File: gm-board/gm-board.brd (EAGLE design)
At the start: 59.5 x 31.5 mm, 61 parts, among them IC1 MCP1700TT, IC2 ZXCT1109, IC3 STM32F030F4, J1 HV_GEN-HOLE, J3 SWD_SHROUD, X1 PKM13EPYH, X2 GM-TUBE

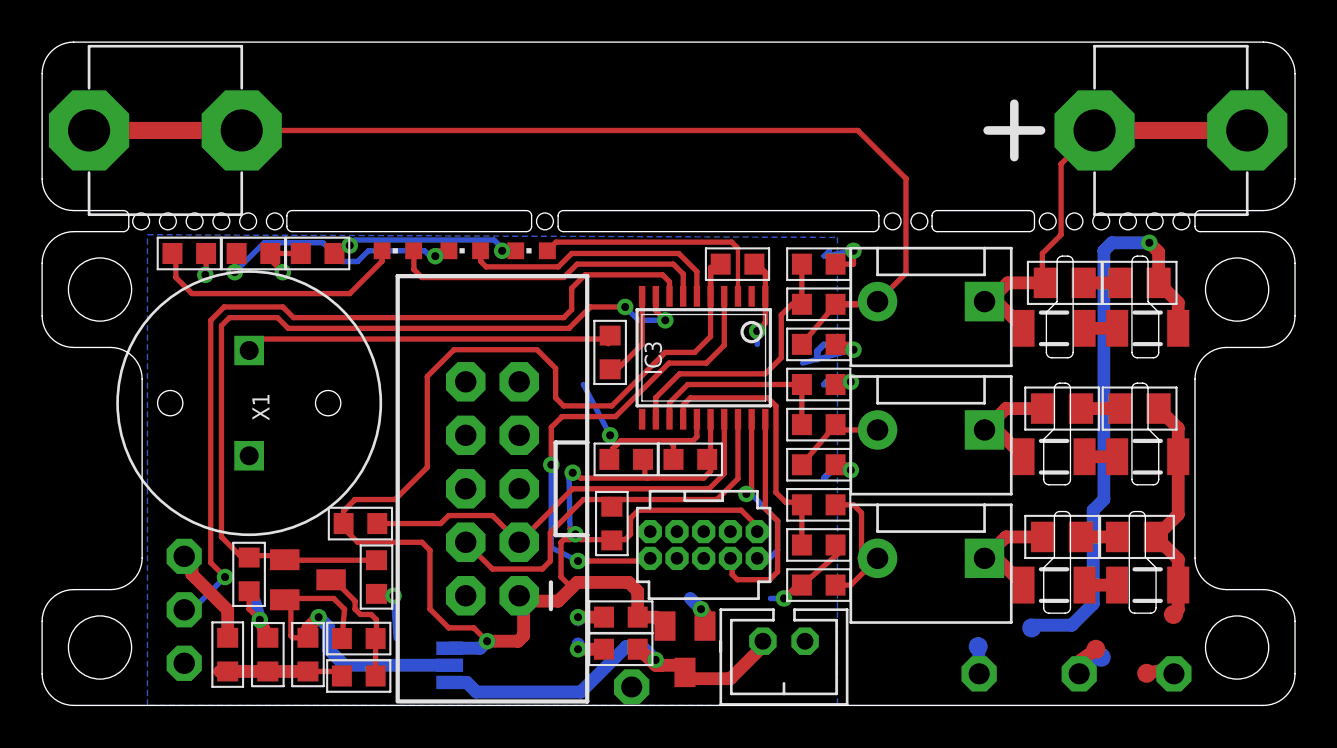
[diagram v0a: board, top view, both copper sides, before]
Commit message: about to panelize
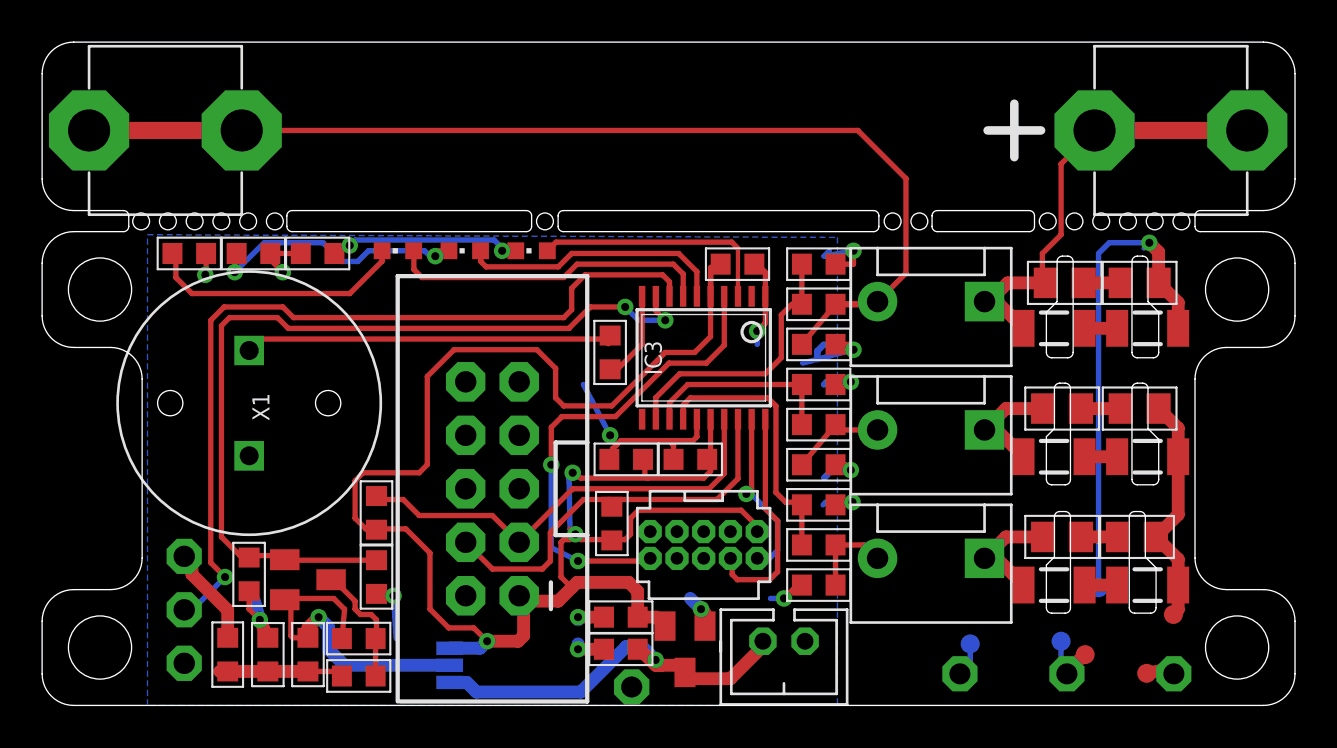
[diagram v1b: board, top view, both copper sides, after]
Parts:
- moved TP5 3.70 mm to (50.4, 5.59)
- moved TP6 2.05 mm to (48.6, 3.05)
- moved C7 1.91 mm to (37.1, 7.62)
- moved R7 1.91 mm to (37.1, 9.53)
- moved R17 0.92 mm to (16.1, 9.14), turned to 270 degrees
- moved TP2 0.57 mm to (49.8, 2.41)
- moved TP3 0.40 mm to (44.3, 2.92)
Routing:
- net N$8: track 27.3 -> 23.5 mm
- net N$9: track 6.80 -> 4.16 mm
- net +3V3: track 85.4 -> 84.8 mm
- net GND: track 45.7 -> 45.1 mm, vias 14 -> 15
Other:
- outline, holes or cut-outs redrawn
